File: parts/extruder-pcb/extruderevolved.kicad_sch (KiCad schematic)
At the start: 8 parts, among them CN1 B-3102R24P-A000, CN2 HC-1.25-2PWT, CN3 HC-1.25-3PWT, CN4 HC-1.25-4PWT, CN5 HC-1.25-5PWT, CN6 X2011WRS-02A-9TSN, CN7 HC-1.25-2PWT, CN8 HC-1.25-2PWT

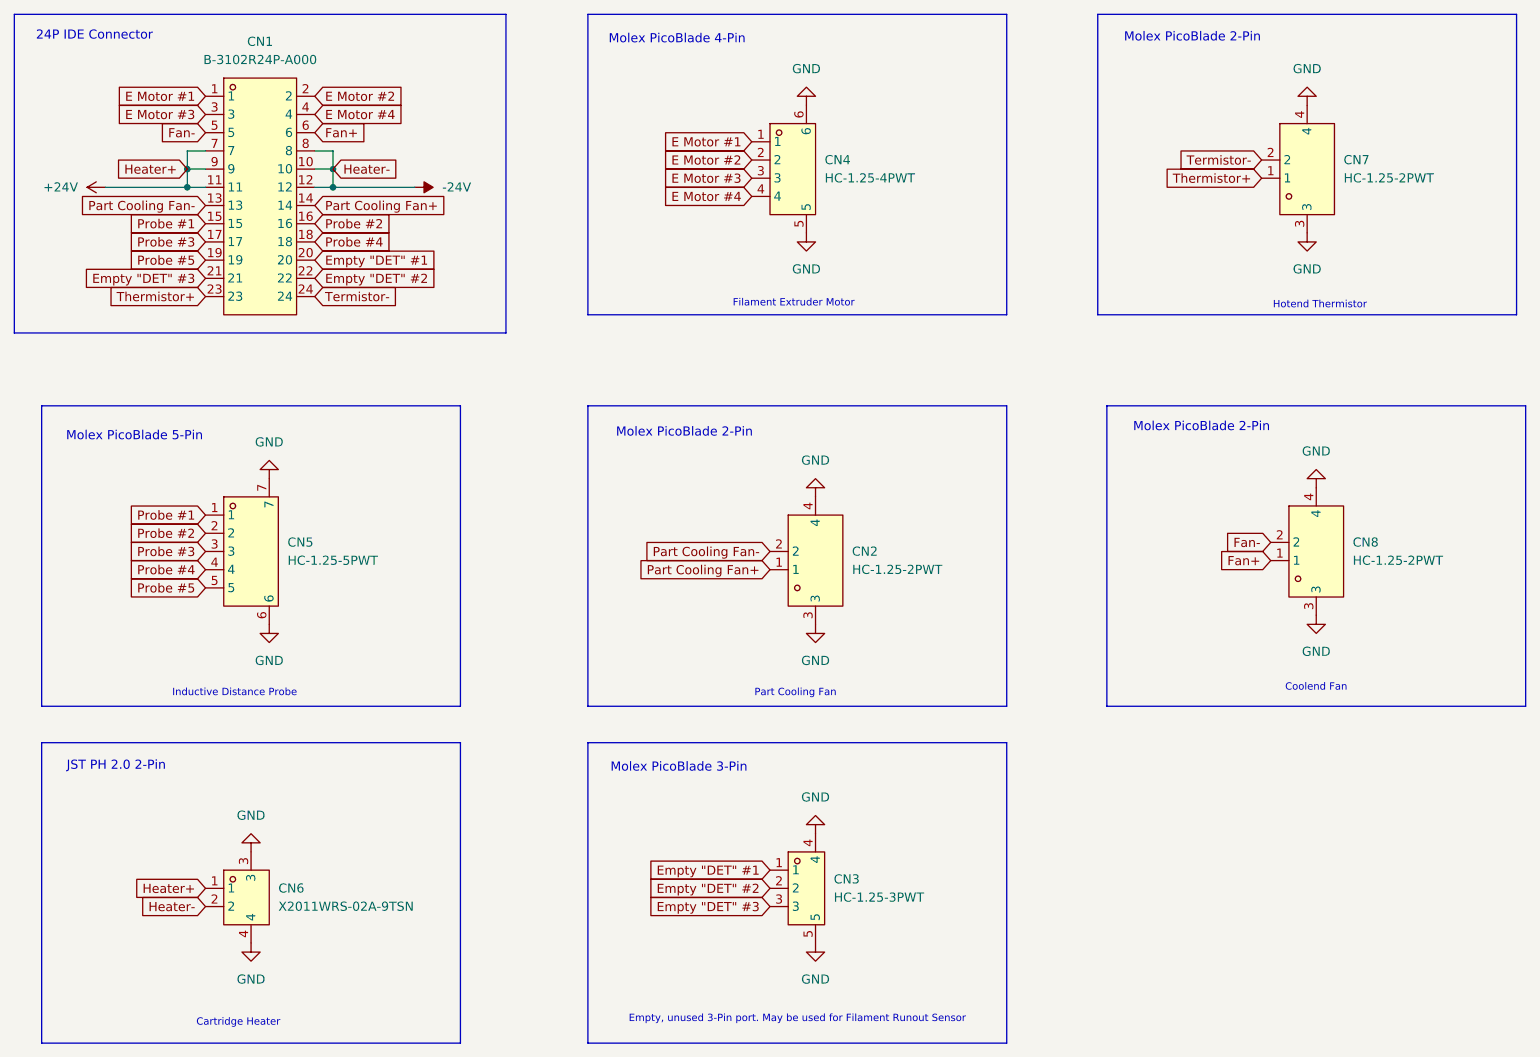
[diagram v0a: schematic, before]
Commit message: upload new PCB files (#51)
* Add files via upload

* Add files via upload
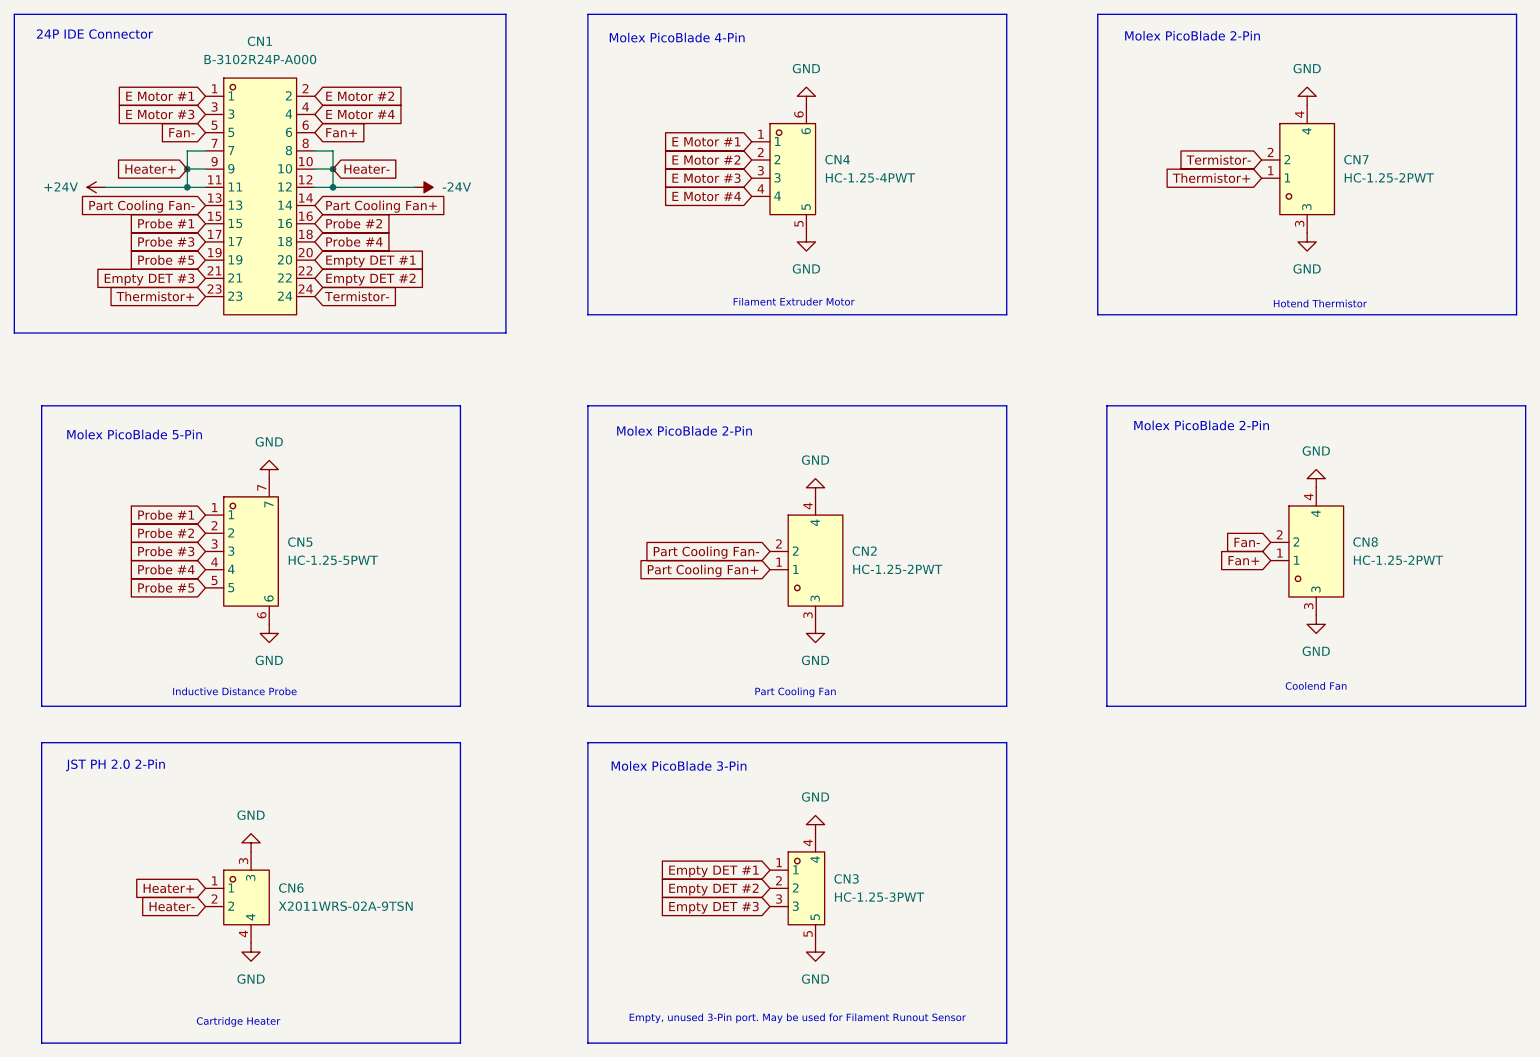
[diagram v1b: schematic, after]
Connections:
- net Empty "DET" #1 renamed Empty DET #1
- net Empty "DET" #2 renamed Empty DET #2
- net Empty "DET" #3 renamed Empty DET #3
